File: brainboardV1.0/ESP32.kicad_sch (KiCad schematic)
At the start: 17 parts, among them J12 Conn_01x03, J13 Conn_01x03, J14 SERIAL1, J15 Conn_01x03, U11 ESP32-WROOM-32D

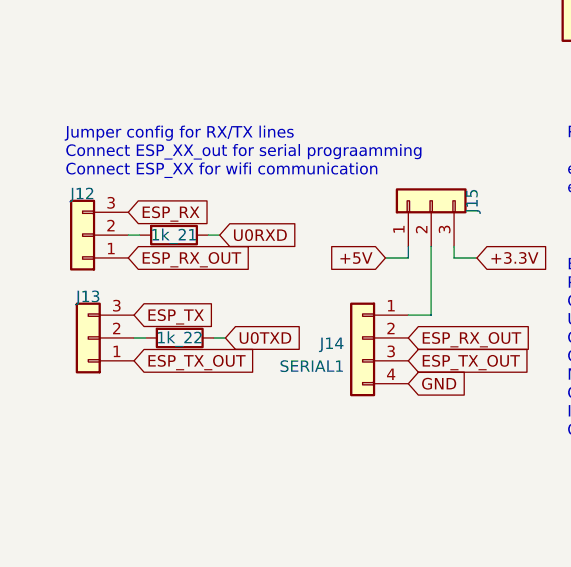
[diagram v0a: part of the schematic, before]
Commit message: finished V1.0
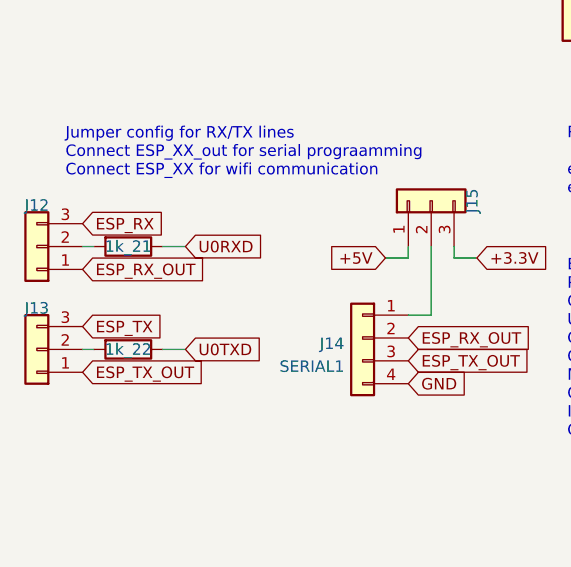
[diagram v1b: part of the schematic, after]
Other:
- moved on the sheet: 1k_21, 1k_22, J12, J13
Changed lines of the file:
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@@
 	(wire
 		(pts
-			(xy 170.18 125.73) (xy 171.45 125.73)
+			(xy 156.21 127) (xy 157.48 127)
 		)
 		(stroke
@@
 	(wire
 		(pts
-			(xy 161.925 137.16) (xy 163.195 137.16)
-		)
-		(stroke
-			(width 0)
-			(type default)
-		)
-	)
-	(wire
-		(pts
 			(xy 200.025 128.27) (xy 197.485 128.27)
 		)
@@
 	(wire
 		(pts
-			(xy 170.815 137.16) (xy 172.085 137.16)
-		)
-		(stroke
-			(width 0)
-			(type default)
-		)
-	)
-	(wire
-		(pts
 			(xy 222.25 30.48) (xy 222.25 35.56)
 		)
@@
 	(wire
 		(pts
+			(xy 156.21 138.43) (xy 157.48 138.43)
+		)
+		(stroke
+			(width 0)
+			(type default)
+		)
+	)
+	(wire
+		(pts
 			(xy 244.475 80.645) (xy 244.475 83.185)
 		)
@@
 	(wire
 		(pts
-			(xy 161.29 125.73) (xy 162.56 125.73)
-		)
-		(stroke
-			(width 0)
-			(type default)
-		)
-	)
-	(wire
-		(pts
 			(xy 194.945 127) (xy 194.945 134.62)
 		)
@@
 	(wire
 		(pts
+			(xy 165.1 138.43) (xy 167.64 138.43)
+		)
+		(stroke
+			(width 0)
+			(type default)
+		)
+	)
+	(wire
+		(pts
 			(xy 175.895 51.435) (xy 187.325 51.435)
 		)
@@
 		(pts
 			(xy 197.485 128.27) (xy 197.485 127)
+		)
+		(stroke
+			(width 0)
+			(type default)
+		)
+	)
+	(wire
+		(pts
+			(xy 165.1 127) (xy 167.64 127)
 		)
 		(stroke
@@
 	(global_label "U0TXD"
 		(shape input)
-		(at 172.085 137.16 0)
+		(at 167.64 138.43 0)
 		(fields_autoplaced yes)
 		(effects
@@
 		)
 		(property "Intersheetrefs" "${INTERSHEET_REFS}"
-			(at 181.0573 137.16 0)
+			(at 176.6123 138.43 0)
 			(effects
 				(font
@@
 	(global_label "ESP_TX_OUT"
 		(shape input)
-		(at 161.925 139.7 0)
+		(at 156.21 140.97 0)
 		(fields_autoplaced yes)
 		(effects
@@
 		)
 		(property "Intersheetrefs" "${INTERSHEET_REFS}"
-			(at 176.2796 139.7 0)
+			(at 170.5646 140.97 0)
 			(effects
 				(font
@@
 	(global_label "ESP_RX"
 		(shape input)
-		(at 161.29 123.19 0)
+		(at 156.21 124.46 0)
 		(fields_autoplaced yes)
 		(effects
@@
 		)
 		(property "Intersheetrefs" "${INTERSHEET_REFS}"
-			(at 171.2714 123.19 0)
+			(at 166.1914 124.46 0)
 			(effects
 				(font
@@
 	(global_label "ESP_RX_OUT"
 		(shape input)
-		(at 161.29 128.27 0)
+		(at 156.21 129.54 0)
 		(fields_autoplaced yes)
 		(effects
@@
 		)
 		(property "Intersheetrefs" "${INTERSHEET_REFS}"
-			(at 175.8676 128.27 0)
+			(at 170.7876 129.54 0)
 			(effects
 				(font
@@
 	(global_label "U0RXD"
 		(shape input)
-		(at 171.45 125.73 0)
+		(at 167.64 127 0)
 		(fields_autoplaced yes)
 		(effects
@@
 		)
 		(property "Intersheetrefs" "${INTERSHEET_REFS}"
-			(at 180.6453 125.73 0)
+			(at 176.8353 127 0)
 			(effects
 				(font
@@
 	(global_label "ESP_TX"
 		(shape input)
-		(at 161.925 134.62 0)
+		(at 156.21 135.89 0)
 		(fields_autoplaced yes)
 		(effects
@@
 		)
 		(property "Intersheetrefs" "${INTERSHEET_REFS}"
-			(at 171.6834 134.62 0)
+			(at 165.9684 135.89 0)
 			(effects
 				(font
@@
 	(symbol
 		(lib_id "Device:R")
-		(at 166.37 125.73 270)
+		(at 161.29 127 270)
 		(unit 1)
 		(exclude_from_sim no)
@@
 		(dnp no)
 		(property "Reference" "1k_21"
-			(at 166.37 125.73 90)
+			(at 161.29 127 90)
 			(effects
 				(font
@@
 		)
 		(property "Value" "1k"
-			(at 166.37 121.92 90)
+			(at 161.29 123.19 90)
 			(effects
 				(font
@@
 		)
 		(property "Footprint" "Resistor_SMD:R_0603_1608Metric"
-			(at 166.37 123.952 90)
+			(at 161.29 125.222 90)
 			(effects
 				(font
@@
 		)
 		(property "Datasheet" "~"
-			(at 166.37 125.73 0)
+			(at 161.29 127 0)
 			(effects
 				(font
@@
 		)
 		(property "Description" ""
-			(at 166.37 125.73 0)
+			(at 161.29 127 0)
 			(effects
 				(font
@@
 		)
 		(property "LCSC" "C25804"
-			(at 166.37 125.73 0)
+			(at 161.29 127 0)
 			(effects
 				(font
@@
 	(symbol
 		(lib_id "Device:R")
-		(at 167.005 137.16 270)
+		(at 161.29 138.43 270)
 		(unit 1)
 		(exclude_from_sim no)
@@
 		(dnp no)
 		(property "Reference" "1k_22"
-			(at 167.005 137.16 90)
+			(at 161.29 138.43 90)
 			(effects
 				(font
@@
 		)
 		(property "Value" "1k"
-			(at 167.005 133.35 90)
+			(at 161.29 134.62 90)
 			(effects
 				(font
@@
 		)
 		(property "Footprint" "Resistor_SMD:R_0603_1608Metric"
-			(at 167.005 135.382 90)
+			(at 161.29 136.652 90)
 			(effects
 				(font
@@
 		)
 		(property "Datasheet" "~"
-			(at 167.005 137.16 0)
+			(at 161.29 138.43 0)
 			(effects
 				(font
@@
 		)
 		(property "Description" ""
-			(at 167.005 137.16 0)
+			(at 161.29 138.43 0)
 			(effects
 				(font
@@
 		)
 		(property "LCSC" "C25804"
-			(at 167.005 137.16 0)
+			(at 161.29 138.43 0)
 			(effects
 				(font
@@
 	(symbol
 		(lib_id "Connector_Generic:Conn_01x03")
-		(at 156.21 125.73 180)
+		(at 151.13 127 180)
 		(unit 1)
 		(exclude_from_sim no)
@@
 		(fields_autoplaced yes)
 		(property "Reference" "J12"
-			(at 156.21 121.158 0)
+			(at 151.13 122.428 0)
 			(effects
 				(font
@@
 		)
 		(property "Value" "Conn_01x03"
-			(at 156.21 121.158 0)
+			(at 151.13 122.428 0)
 			(effects
 				(font
@@
 		)
 		(property "Footprint" "Connector_PinHeader_2.54mm:PinHeader_1x03_P2.54mm_Vertical"
-			(at 156.21 125.73 0)
+			(at 151.13 127 0)
 			(effects
 				(font
@@
 		)
 		(property "Datasheet" "~"
-			(at 156.21 125.73 0)
+			(at 151.13 127 0)
 			(effects
 				(font
@@
 		)
 		(property "Description" ""
-			(at 156.21 125.73 0)
+			(at 151.13 127 0)
 			(effects
 				(font
@@
 	(symbol
 		(lib_id "Connector_Generic:Conn_01x03")
-		(at 156.845 137.16 180)
+		(at 151.13 138.43 180)
 		(unit 1)
 		(exclude_from_sim no)
@@
 		(fields_autoplaced yes)
 		(property "Reference" "J13"
-			(at 156.845 132.588 0)
+			(at 151.13 133.858 0)
 			(effects
 				(font
@@
 		)
 		(property "Value" "Conn_01x03"
-			(at 156.845 132.588 0)
+			(at 151.13 133.858 0)
 			(effects
 				(font
@@
 		)
 		(property "Footprint" "Connector_PinHeader_2.54mm:PinHeader_1x03_P2.54mm_Vertical"
-			(at 156.845 137.16 0)
+			(at 151.13 138.43 0)
 			(effects
 				(font
@@
 		)
 		(property "Datasheet" "~"
-			(at 156.845 137.16 0)
+			(at 151.13 138.43 0)
 			(effects
 				(font
@@
 		)
 		(property "Description" ""
-			(at 156.845 137.16 0)
-			(effects
-				(font
+			(at 151.13 138.43 0)
+			(effects
+				(font
